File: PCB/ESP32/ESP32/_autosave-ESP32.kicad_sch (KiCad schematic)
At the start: 31 parts, among them J1 Camera_Receptacle_THT, J1 Conn_01x02_Pin, J1 USB_B_Micro, J2 Conn_01x02_Socket, SW1 RESET, SW2 BOOT, SW3 LRA Switch, U1 DRV2605LTDGSRQ1, U1 ESP32-S2-SOLO-U-N4, U1 MCP73832T-2ACI/OT

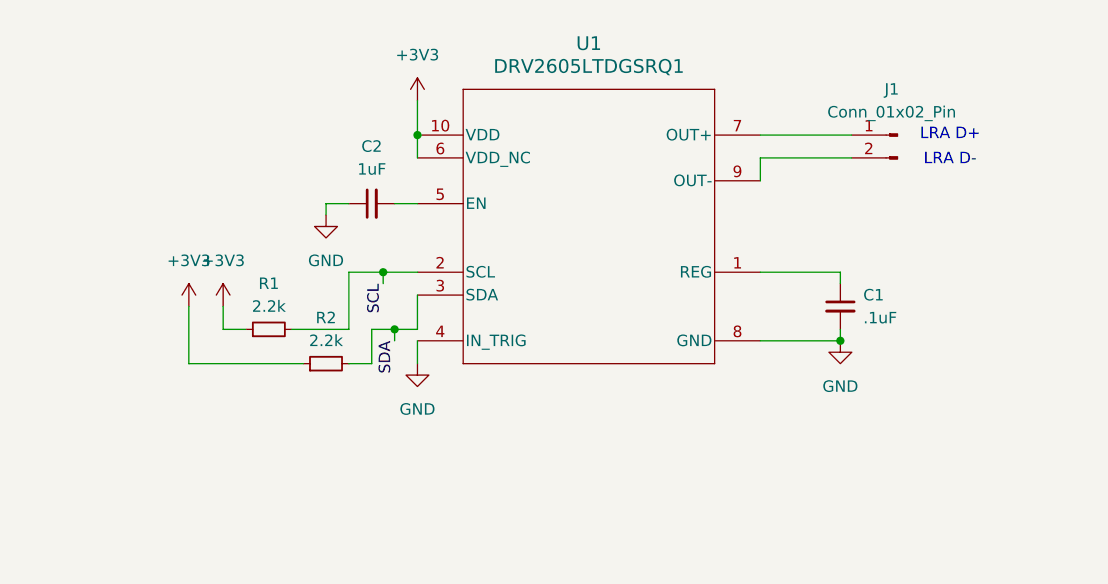
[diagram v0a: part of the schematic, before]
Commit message: Layout
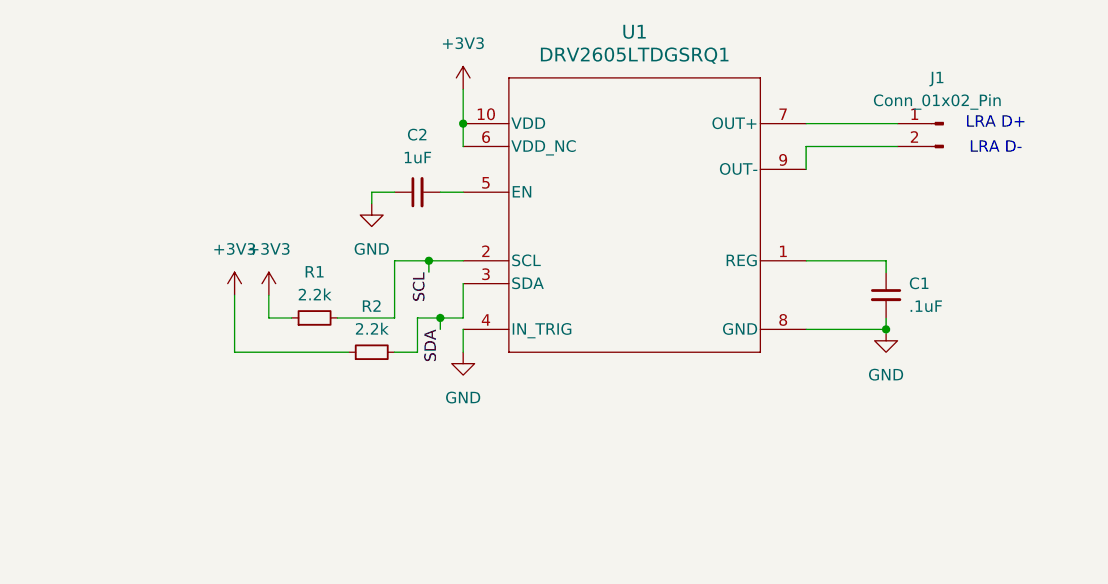
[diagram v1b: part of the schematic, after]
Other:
- moved on the sheet: C1, C2, J1, R1, R2, U1
